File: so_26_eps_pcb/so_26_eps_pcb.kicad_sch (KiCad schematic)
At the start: 47 parts, among them J1 Conn_02x12_Odd_Even, J3 Conn_01x02, SW1 SW_SPDT, U1 LM22679TJ-ADJ/NOPB, U2 LM22679TJ-ADJ/NOPB

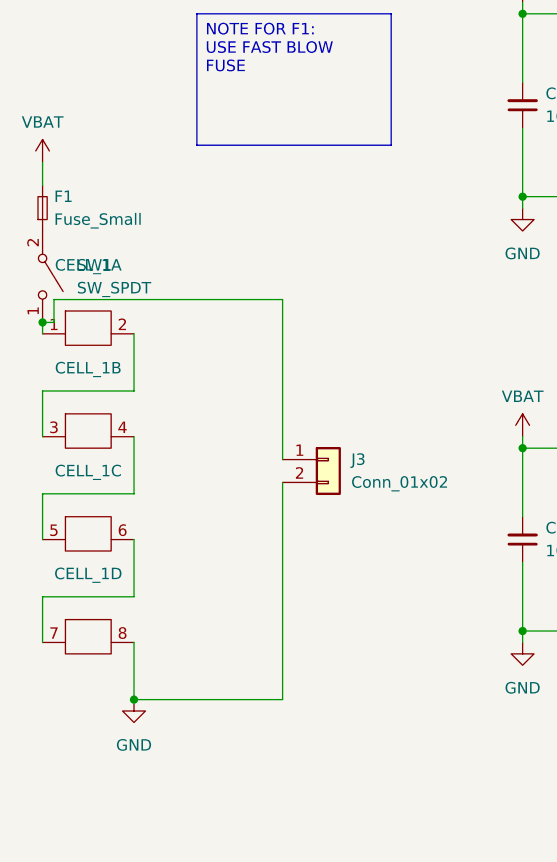
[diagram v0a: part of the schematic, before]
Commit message: added text
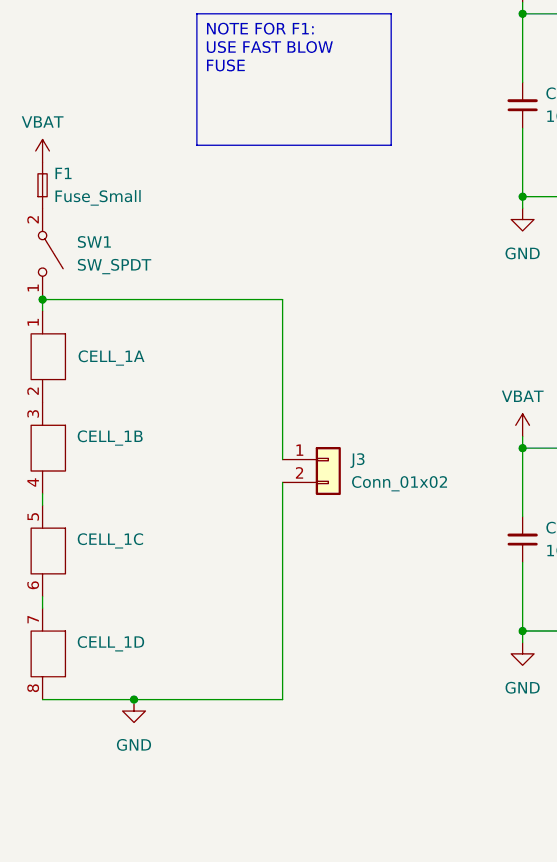
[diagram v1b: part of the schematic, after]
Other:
- moved on the sheet: CELL_1A, CELL_1B, CELL_1C, CELL_1D, F1, SW1
